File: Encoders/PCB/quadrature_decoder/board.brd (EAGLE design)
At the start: 160 x 100 mm, 14 parts

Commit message: Revert "deleted temp eagle files"
This reverts commit 96ff2f756feb4d77b0f38149fa13669738a3dee2.
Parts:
- moved SV7 333.3 mm to (-139.7, -226.1)
- moved U$5 320.3 mm to (-146.1, -241.3)
- moved U$4 294.4 mm to (-146.1, -210.8)
- moved SV6 280.3 mm to (-139.7, -195.6)
- moved U$3 270.0 mm to (-146.1, -180.3)
- moved SV5 254.6 mm to (-139.7, -165.1)
- moved U$2 247.7 mm to (-146.1, -149.9)
- moved SV4 231.0 mm to (-139.7, -134.6)
- moved U$1 227.9 mm to (-146.1, -119.4)
- moved SV3 210.0 mm to (-139.7, -104.1)
- moved SV2 205.0 mm to (-142.2, -88.9)
- moved SV1 192.6 mm to (-139.7, -73.7)
- moved U$7 104.4 mm to (62.2, 43.2)
- moved U$6 88.9 mm to (-146.1, 7.62)
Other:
- board size 160 x 100 mm -> 608.3 x 423.8 mm

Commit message: new board layout
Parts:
- removed SV1, SV3, SV4, SV5, SV6, SV7: (no value), con-lstb:MA05-1
- removed SV2: (no value), con-lstb:MA03-1
- removed U$1, U$2, U$3, U$4, U$5, U$6: LFLS7366R, encoder_project:SO14
- added CON1, CON2, CON3, CON4, CON5, CON6: (no value), con-lstb:MA05-1
- added IC1, IC2, IC3, IC4, IC5, IC6: LFLS7366R, encoder_project:SO14
- added UART: (no value), con-lstb:MA03-1
- moved U$7 20.3 mm to (62.2, 22.9)
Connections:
- net 3.3V: now also IC1.14, IC2.14, IC3.14, IC4.14, IC5.14, IC6.14; no longer U$1.14, U$2.14, U$3.14, U$4.14, U$5.14, U$6.14
- net 5V: now also CON1.4, CON2.4, CON3.4, CON4.4, CON5.4, CON6.4; no longer SV1.4, SV3.4, SV4.4, SV5.4, SV6.4, SV7.4
- net FCKI: now also IC1.2, IC2.2, IC3.2, IC4.2, IC5.2, IC6.2; no longer U$1.2, U$2.2, U$3.2, U$4.2, U$5.2, U$6.2
- net GND: now also UART.1; no longer SV2.1
- net MISO: now also IC1.6, IC2.6, IC3.6, IC4.6, IC5.6, IC6.6; no longer U$1.6, U$2.6, U$3.6, U$4.6, U$5.6, U$6.6
- net MOSI: now also IC1.7, IC2.7, IC3.7, IC4.7, IC5.7, IC6.7; no longer U$1.7, U$2.7, U$3.7, U$4.7, U$5.7, U$6.7
- net N$1: now also CON2.1, IC2.3; no longer SV1.1, U$6.3
- net N$10: now also CON3.5, IC3.11; no longer SV3.5, U$1.11
- net N$11: now also CON1.1, IC1.3; no longer SV4.1, U$2.3
- net N$12: now also CON1.2, IC1.10; no longer SV4.2, U$2.10
- net N$13: now also CON1.3, IC1.12; no longer SV4.3, U$2.12
- net N$14: now also CON1.5, IC1.11; no longer SV4.5, U$2.11
- net N$15: now also CON5.1, IC5.3; no longer SV5.1, U$3.3
- net N$16: now also CON5.2, IC5.10; no longer SV5.2, U$3.10
- net N$17: now also CON5.3, IC5.12; no longer SV5.3, U$3.12
- net N$18: now also CON5.5, IC5.11; no longer SV5.5, U$3.11
- net N$19: now also CON6.1, IC6.3; no longer SV6.1, U$4.3
- net N$2: now also CON2.2, IC2.10; no longer SV1.2, U$6.10
- net N$20: now also CON6.2, IC6.10; no longer SV6.2, U$4.10
- net N$21: now also CON6.3, IC6.12; no longer SV6.3, U$4.12
- net N$22: now also CON6.5, IC6.11; no longer SV6.5, U$4.11
- net N$23: now also CON4.1, IC4.3; no longer SV7.1, U$5.3
- net N$24: now also CON4.2, IC4.10; no longer SV7.2, U$5.10
- net N$25: now also CON4.3, IC4.12; no longer SV7.3, U$5.12
- net N$26: now also CON4.5, IC4.11; no longer SV7.5, U$5.11
- net N$3: now also UART.3; no longer SV2.3
- net N$4: now also UART.2; no longer SV2.2
- net N$5: now also CON2.3, IC2.12; no longer SV1.3, U$6.12
- net N$6: now also CON3.1, IC3.3; no longer SV3.1, U$1.3
- net N$7: now also CON2.5, IC2.11; no longer SV1.5, U$6.11
- net N$8: now also CON3.2, IC3.10; no longer SV3.2, U$1.10
- net N$9: now also CON3.3, IC3.12; no longer SV3.3, U$1.12
- net SCK: now also IC1.5, IC2.5, IC3.5, IC4.5, IC5.5, IC6.5; no longer U$1.5, U$2.5, U$3.5, U$4.5, U$5.5, U$6.5
- net SS1: now also IC1.4; no longer U$2.4
- net SS2: now also IC2.4; no longer U$6.4
- net SS3: now also IC3.4; no longer U$1.4
- net SS4: now also IC4.4; no longer U$5.4
- net SS5: now also IC5.4; no longer U$3.4
- net SS6: now also IC6.4; no longer U$4.4
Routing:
- net FCKI: track 0.00 -> 152.4 mm, vias 0 -> 4
- net SCK: track 0.00 -> 133.3 mm, vias 0 -> 6
- net 3.3V: track 0.00 -> 126.6 mm, vias 0 -> 6
- net 5V: track 0.00 -> 125.5 mm
- net MISO: track 0.00 -> 120.1 mm, vias 0 -> 4
- net SS6: track 0.00 -> 118.6 mm
- net MOSI: track 0.00 -> 116.3 mm, vias 0 -> 5
- net SS1: track 0.00 -> 99.4 mm
- net SS2: track 0.00 -> 92.1 mm
- net SS3: track 0.00 -> 51.8 mm, vias 0 -> 1
- net SS5: track 0.00 -> 39.0 mm, vias 0 -> 3
- net N$12: track 0.00 -> 28.6 mm
- net N$4: track 0.00 -> 25.9 mm
- net N$3: track 0.00 -> 25.2 mm
- net N$2: track 0.00 -> 24.4 mm, vias 0 -> 1
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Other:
- board size 608.3 x 423.8 mm -> 84.8 x 55.9 mm

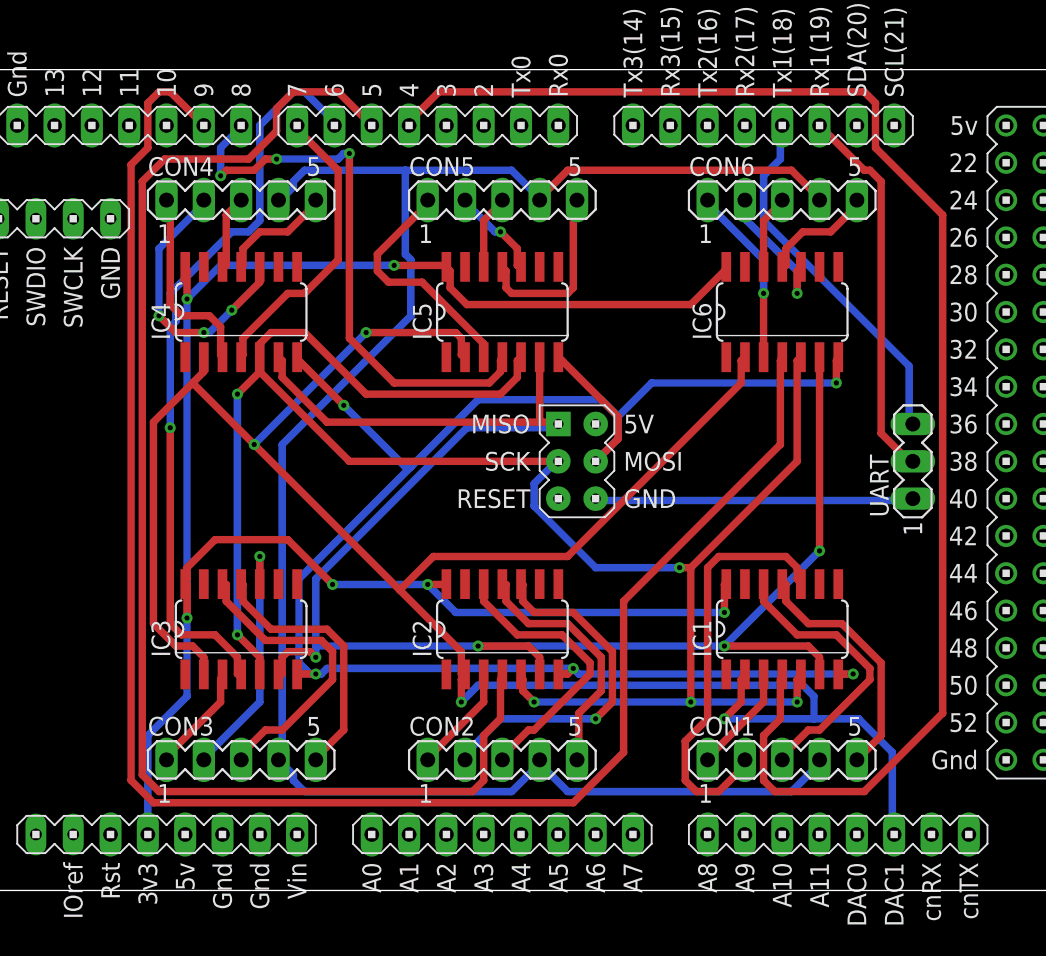
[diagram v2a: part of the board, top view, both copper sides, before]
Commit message: new board
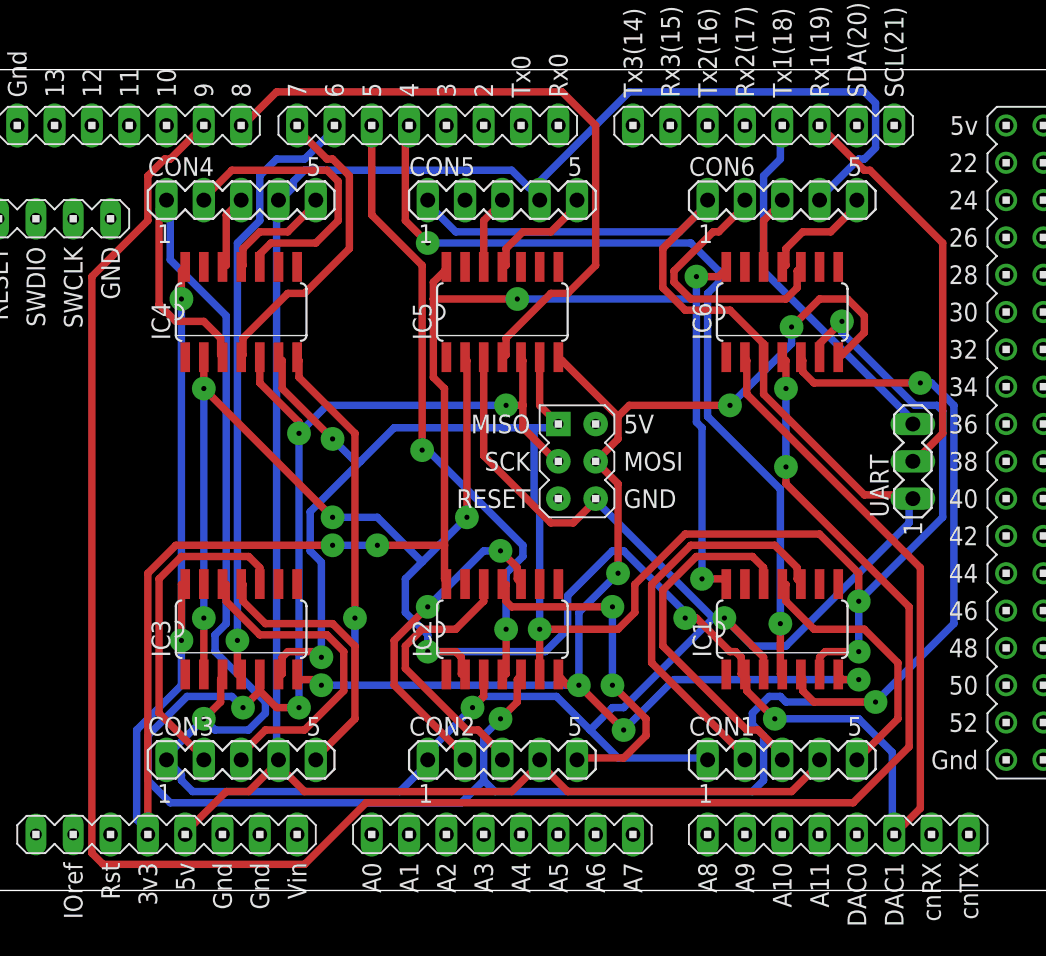
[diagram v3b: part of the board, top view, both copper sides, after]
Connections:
- removed net N$1: CON2.1, IC2.3
- removed net N$11: CON1.1, IC1.3
- removed net N$15: CON5.1, IC5.3
- removed net N$19: CON6.1, IC6.3
- removed net N$23: CON4.1, IC4.3
- removed net N$6: CON3.1, IC3.3
- net 5V: now also U$7.5V
- net GND: now also CON1.1, CON2.1, CON3.1, CON4.1, CON5.1, CON6.1, IC1.3, IC2.3, IC3.3, IC4.3, IC5.3, IC6.3
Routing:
- net GND: track 21.7 -> 227.7 mm, vias 0 -> 3
- net SS2: track 92.1 -> 42.6 mm, vias 0 -> 2
- net SS1: track 99.4 -> 59.4 mm, vias 0 -> 2
- net SCK: track 133.3 -> 173.0 mm, vias 6 -> 7
- net SS6: track 118.6 -> 142.3 mm, vias 0 -> 2
- net 3.3V: track 126.6 -> 148.3 mm, vias 6 -> 7
- net 5V: track 125.5 -> 142.1 mm
- net N$15: track 16.5 -> 0.00 mm
- net N$23: track 13.4 -> 0.00 mm
- net N$19: track 12.3 -> 0.00 mm, vias 1 -> 0
- net SS3: track 51.8 -> 41.8 mm
- net MISO: track 120.1 -> 129.8 mm, vias 4 -> 6
- net N$20: track 9.70 -> 18.6 mm, vias 1 -> 0
- net N$6: track 7.47 -> 0.00 mm
- net N$1: track 7.39 -> 0.00 mm
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
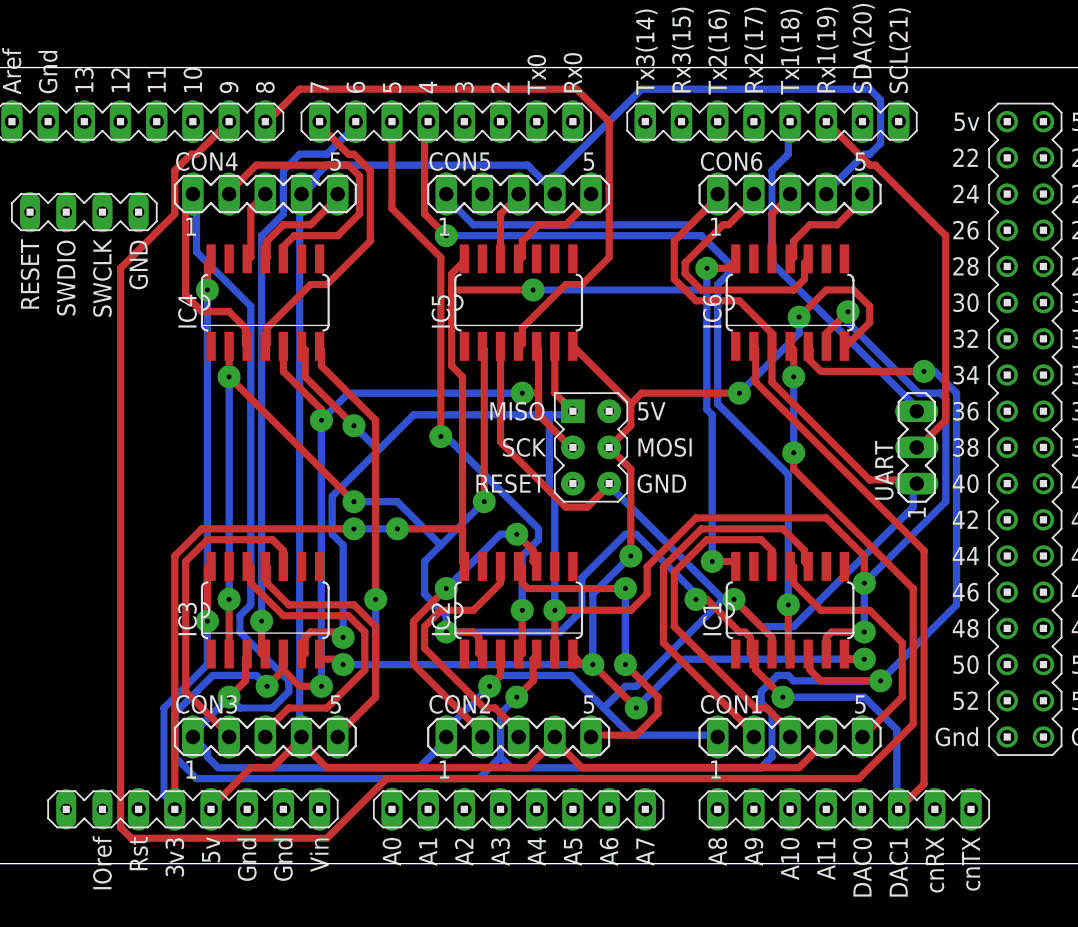
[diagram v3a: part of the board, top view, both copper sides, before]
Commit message: another board
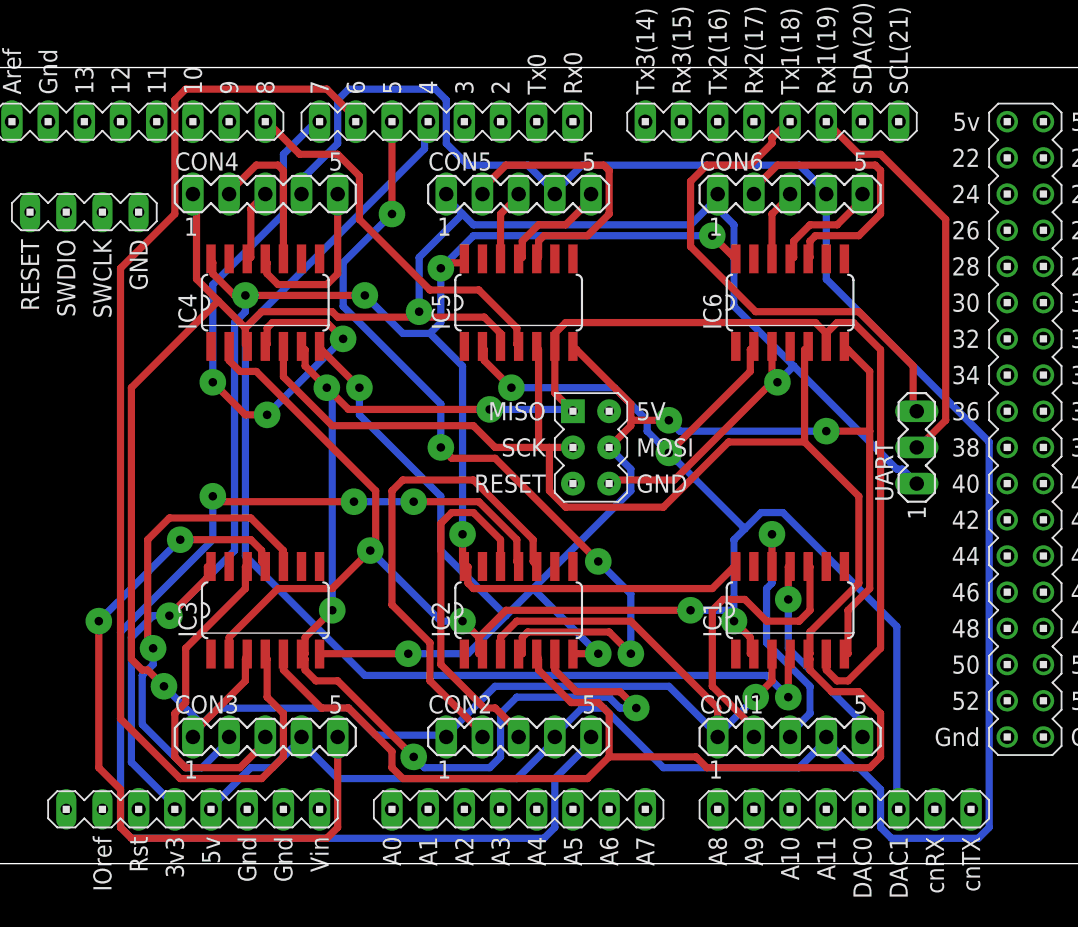
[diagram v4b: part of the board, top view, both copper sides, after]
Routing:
- net SS6: track 142.3 -> 0.00 mm, vias 2 -> 0
- net N$7: track 23.9 -> 89.0 mm, vias 2 -> 3
- net SS3: track 41.8 -> 81.0 mm, vias 1 -> 0
- net N$10: track 19.0 -> 52.6 mm, vias 0 -> 2
- net SCK: track 173.0 -> 148.7 mm, vias 7 -> 0
- net 5V: track 142.1 -> 165.9 mm
- net SS1: track 59.4 -> 81.2 mm, vias 2 -> 1
- net N$16: track 0.00 -> 20.5 mm
- net SS4: track 21.5 -> 41.1 mm, vias 0 -> 3
- net FCKI: track 154.3 -> 135.0 mm, vias 7 -> 6
- net SS5: track 45.1 -> 26.8 mm
- net 3.3V: track 148.3 -> 131.7 mm, vias 7 -> 6
- net SS2: track 42.6 -> 58.7 mm, vias 2 -> 4
- net N$8: track 22.5 -> 34.0 mm, vias 0 -> 1
- net N$2: track 22.8 -> 33.9 mm, vias 2 -> 0
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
